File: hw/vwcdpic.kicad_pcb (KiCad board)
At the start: 2 copper layers, 14.6 x 13.1 mm, 12 parts, among them U1 PIC12F629, U2 LM78L05ACZ, U3 MC78L05ACH

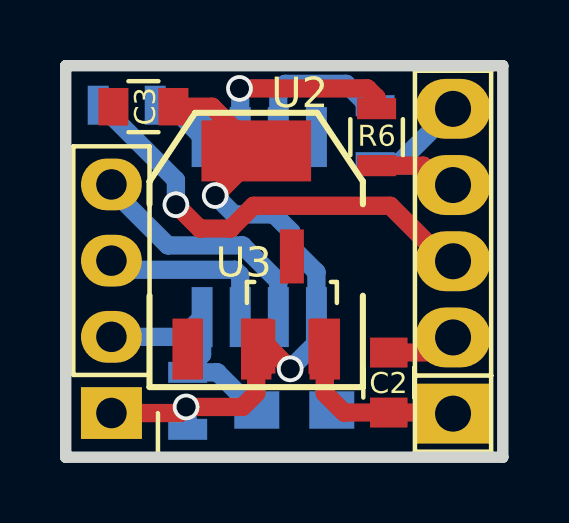
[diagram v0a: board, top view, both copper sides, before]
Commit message: hw and pictures changes
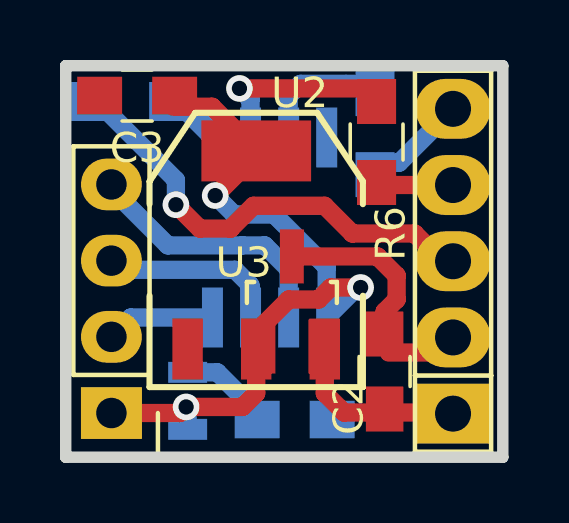
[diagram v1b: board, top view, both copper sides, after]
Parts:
- C2, C3: footprint Capacitors_SMD:C_0805 -> Capacitors_SMD:C_0805_HandSoldering
- R5, R6, R7: footprint Resistors_SMD:R_0805 -> Resistors_SMD:R_0805_HandSoldering
- moved C3 0.43 mm to (140.2, 115.4)
- moved C2 0.39 mm to (148.4, 124.6)
- moved U1 0.34 mm to (144.6, 119.8)
- moved C1 0.32 mm to (145.4, 126.2)
- moved R7 0.19 mm to (139.9, 115.6)
- moved R6 0.16 mm to (148.1, 117.0)
- renumbered RADIO1 to RADIO
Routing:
- net GND: track 2.41 -> 8.28 mm
- net +5V: track 23.5 -> 26.6 mm
- net Net-(R5-Pad1): track 5.17 -> 4.57 mm
- net ARCHOS: track 8.85 -> 9.44 mm
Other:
- net class Default: via_drill 0.635 -> 0.508
